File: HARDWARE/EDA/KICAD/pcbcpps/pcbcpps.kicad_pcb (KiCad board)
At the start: 2 copper layers, 57.5 x 38.5 mm, 20 parts, among them J1 LINE IN, J10 0V, J11 EARTH, J12 EARTH, J2 NEUTRAL, J3 +12V, J4 0V, J5 LINE OUT, J6 LINE OUT, J7 NEUTRAL, J9 +12V

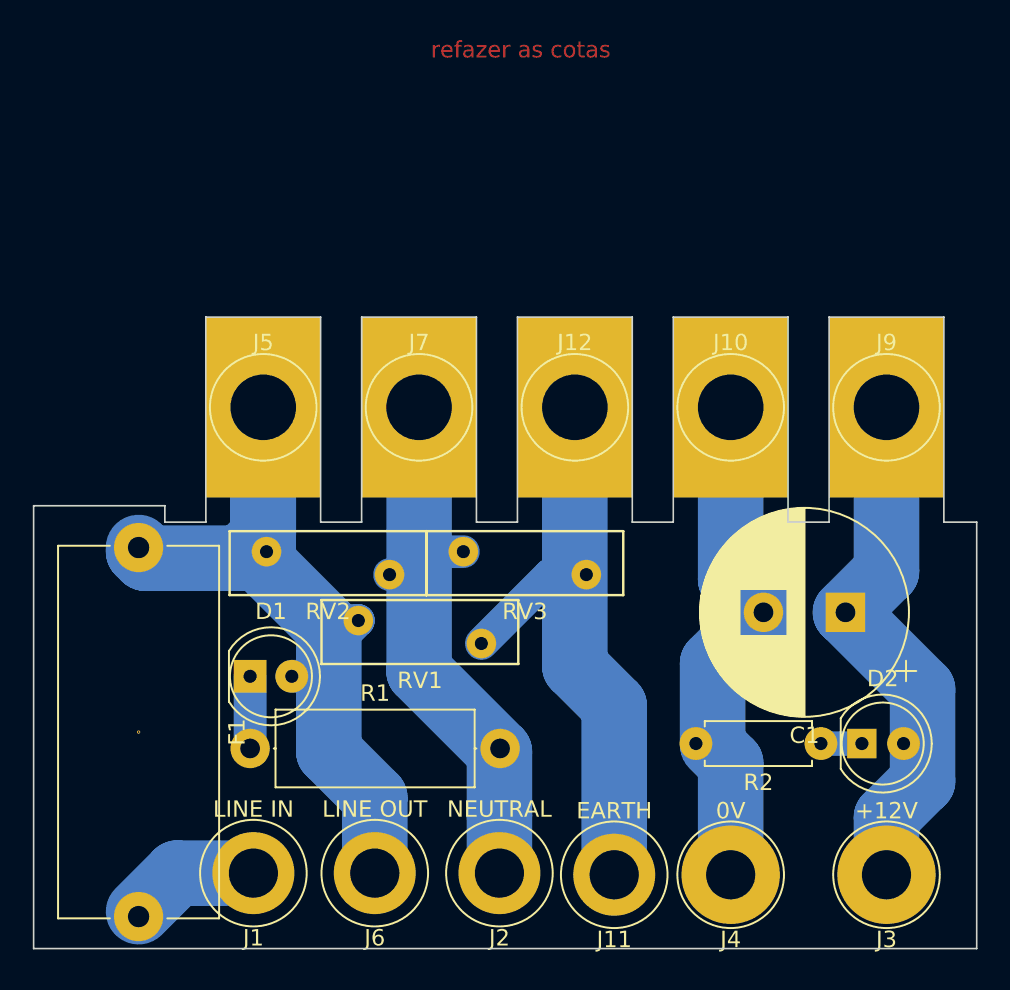
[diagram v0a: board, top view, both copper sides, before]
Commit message: adjust pcb
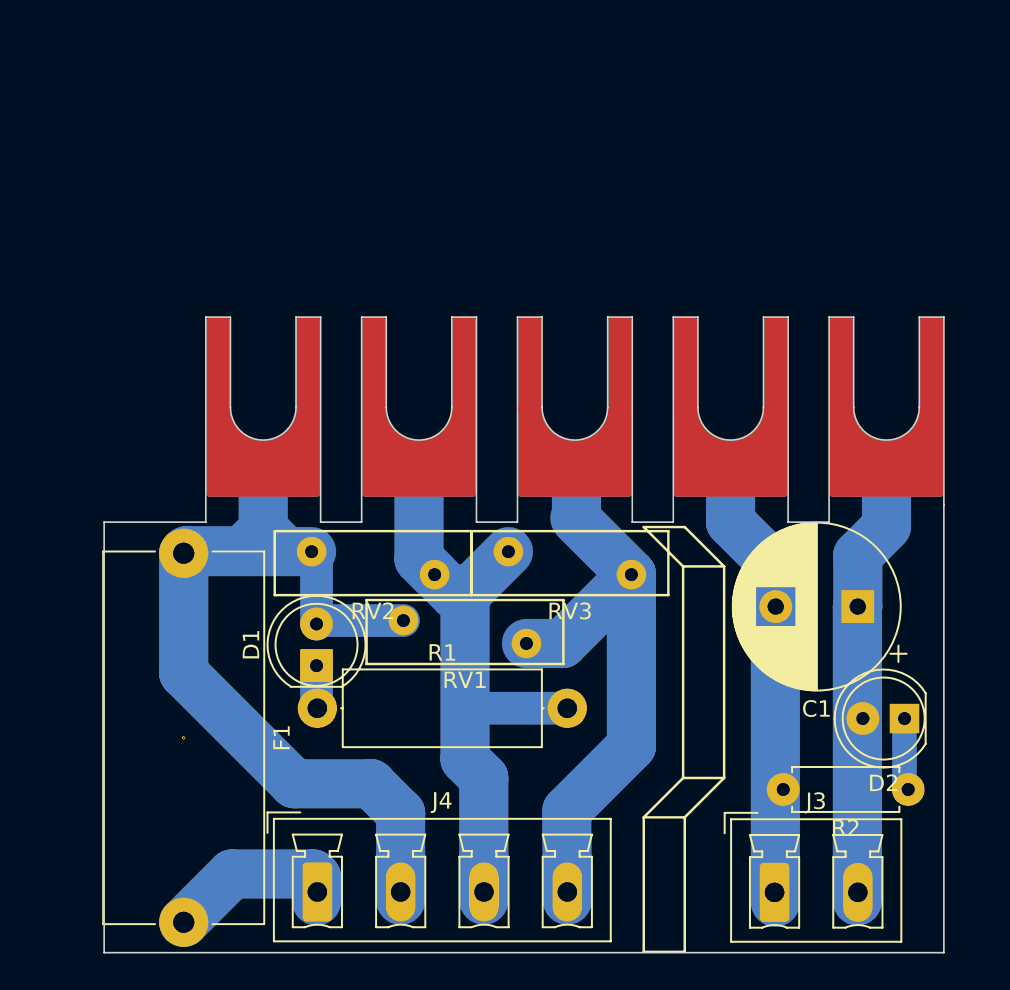
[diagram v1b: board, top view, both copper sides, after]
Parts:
- removed J1: LINE IN, TestPoint:TestPoint_Plated_Hole_D5.0mm
- removed J10: 0V, TestPoint:TestPoint_Plated_Hole_D5.0mm
- removed J11, J12: EARTH, TestPoint:TestPoint_Plated_Hole_D5.0mm
- removed J2, J7: NEUTRAL, TestPoint:TestPoint_Plated_Hole_D5.0mm
- removed J5, J6: LINE OUT, TestPoint:TestPoint_Plated_Hole_D5.0mm
- removed J9: +12V, TestPoint:TestPoint_Plated_Hole_D5.0mm
- C1: footprint Capacitor_THT:CP_Radial_D12.5mm_P5.00mm -> Capacitor_THT:CP_Radial_D10.0mm_P5.00mm
- J3: value +12V -> PWR; footprint TestPoint:TestPoint_Plated_Hole_D5.0mm -> Connector_Phoenix_MC_HighVoltage:PhoenixContact_MCV_1,5_2-G-5.08_1x02_P5.08mm_Vertical
- J4: value 0V -> PWR; footprint TestPoint:TestPoint_Plated_Hole_D5.0mm -> Connector_Phoenix_MC_HighVoltage:PhoenixContact_MCV_1,5_4-G-5.08_1x04_P5.08mm_Vertical
- moved J4 25.2 mm to (137.9, 113.2), turned to 0 degrees
- moved J3 6.91 mm to (165.8, 113.3), turned to 0 degrees
- moved R2 6.02 mm to (173.9, 107.0)
- moved R1 4.78 mm to (137.9, 102.0)
- moved D1 4.10 mm to (137.8, 99.5), turned to 90 degrees
- moved D2 3.01 mm to (173.7, 102.7), turned to 180 degrees
- moved F1 2.77 mm to (129.8, 92.6)
- moved RV1 2.75 mm to (143.2, 96.7)
- moved RV2 2.75 mm to (137.6, 92.5)
- moved RV3 2.75 mm to (149.6, 92.5)
- moved C1 0.83 mm to (170.8, 95.8)
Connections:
- C1 pad 2: Net-(C1-Pad2) -> GND
- D1 pad 2: Net-(D1-Pad2) -> /LINE_OUT
- F1 pad 1: Net-(D1-Pad2) -> /LINE_OUT
- J3 pad 1: Net-(C1-Pad1) -> GND
- J4 pad 1: Net-(C1-Pad2) -> Net-(F1-Pad2)
- R1 pad 2: Net-(J2-Pad1) -> Net-(J4-Pad3)
- R2 pad 2: Net-(C1-Pad2) -> GND
- RV1 pad 1: Net-(D1-Pad2) -> /LINE_OUT
- RV1 pad 2: Net-(J11-Pad1) -> Net-(J12-Pad1)
- RV2 pad 1: Net-(D1-Pad2) -> /LINE_OUT
- RV2 pad 2: Net-(J2-Pad1) -> Net-(J4-Pad3)
- RV3 pad 1: Net-(J2-Pad1) -> Net-(J4-Pad3)
- RV3 pad 2: Net-(J11-Pad1) -> Net-(J12-Pad1)
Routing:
- net /LINE_OUT: track 0.00 -> 64.7 mm
- net Net-(D1-Pad2): track 60.2 -> 0.00 mm
- net Net-(J4-Pad3): track 0.00 -> 44.4 mm
- net Net-(J12-Pad1): track 0.00 -> 40.6 mm
- net Net-(J11-Pad1): track 37.6 -> 0.00 mm
- net Net-(J2-Pad1): track 35.5 -> 0.00 mm
- net Net-(C1-Pad2): track 31.0 -> 0.00 mm
- net GND: track 0.00 -> 25.9 mm
- net Net-(C1-Pad1): track 32.4 -> 25.4 mm
- net Net-(F1-Pad2): track 16.1 -> 10.9 mm
- net Net-(D2-Pad1): track 2.50 -> 4.42 mm
- net Net-(D1-Pad1): track 4.40 -> 2.62 mm
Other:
- board size 57.5 x 38.5 mm -> 51.2 x 38.8 mm
- board text removed: "refazer as cotas"
